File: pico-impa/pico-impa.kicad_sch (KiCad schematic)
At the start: 12 parts, among them J1 Barrel_Jack_MountingPin, U1 Pico, U2 Pico, U3 AMS1117-3.3

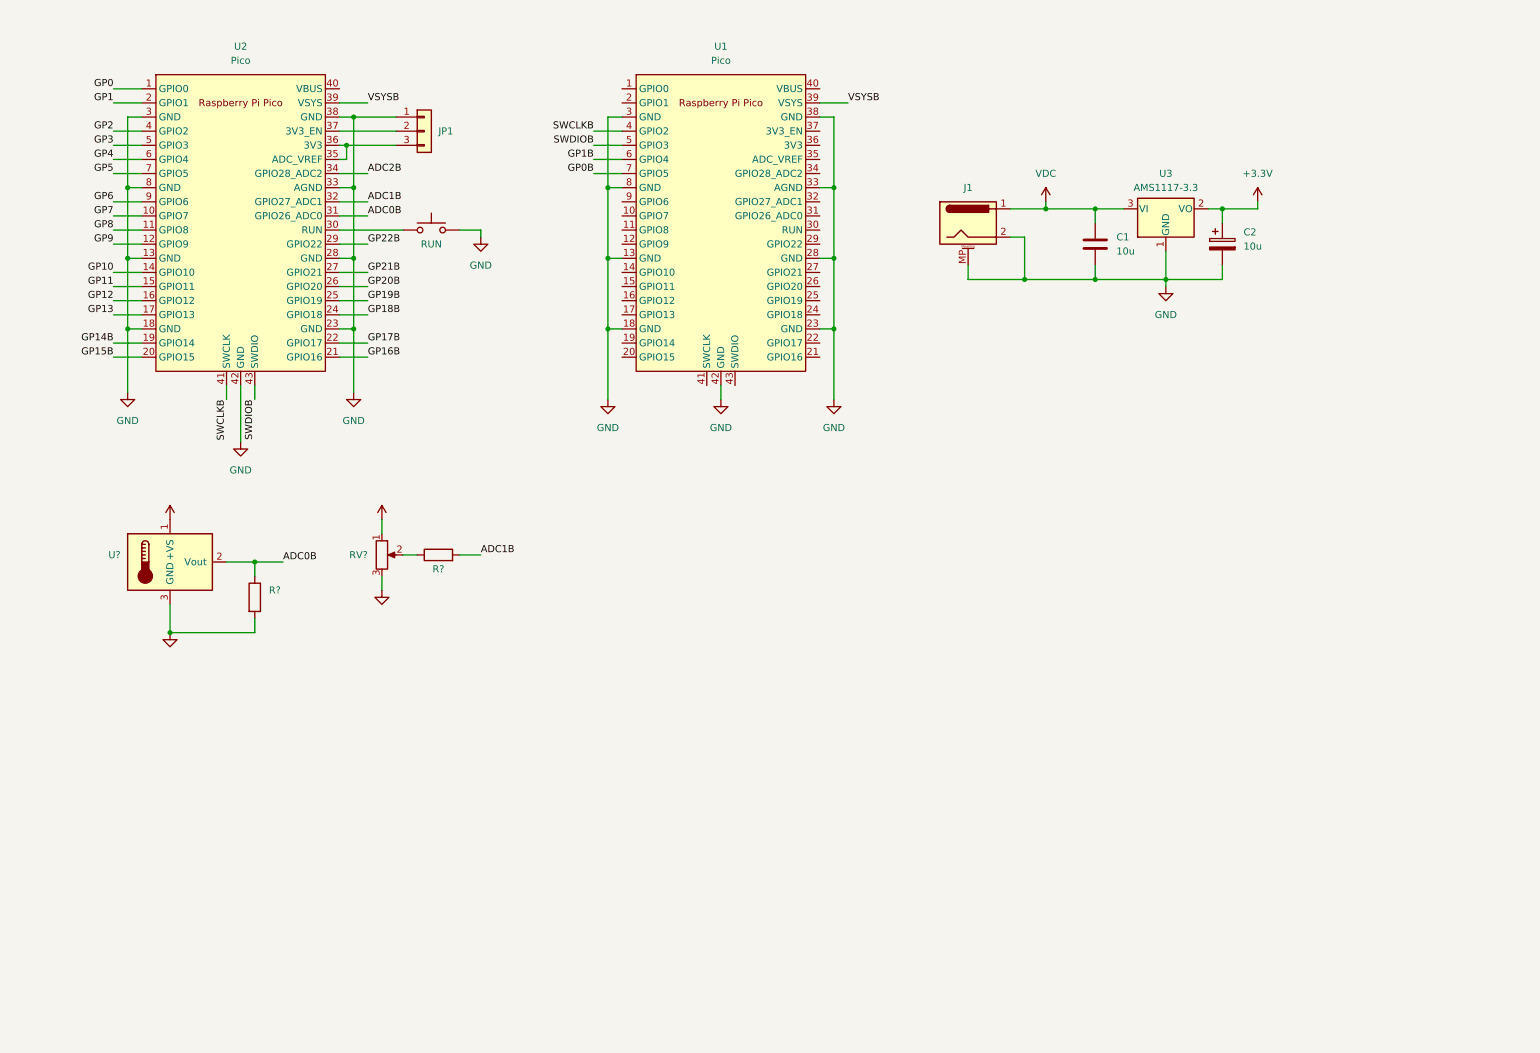
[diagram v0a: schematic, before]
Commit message: feat: first schematic version
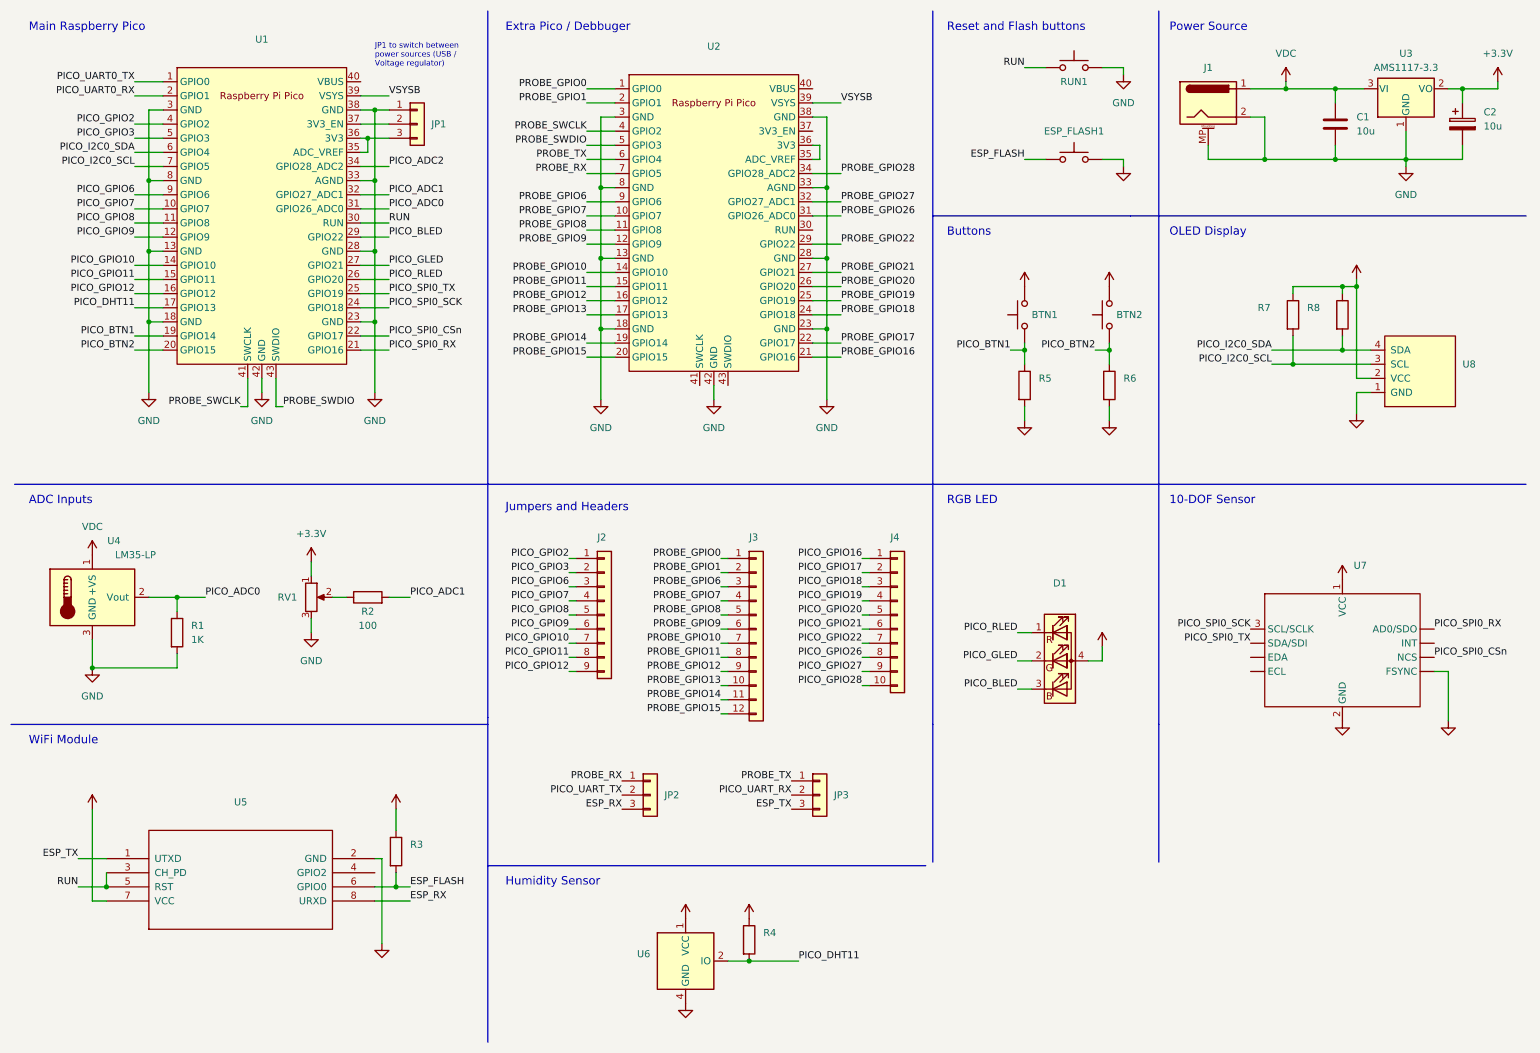
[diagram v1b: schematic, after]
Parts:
- added BTN1, BTN2, ESP_FLASH1: (no value), symbol Switch:SW_Push
- added D1: (no value), symbol Device:LED_RGBA
- added J2: (no value), symbol Connector_Generic:Conn_01x09
- added J3: (no value), symbol Connector_Generic:Conn_01x12
- added J4: (no value), symbol Connector_Generic:Conn_01x10
- added JP2, JP3: (no value), symbol Connector_Generic:Conn_01x03
- added R3, R4, R5, R6, R7, R8: (no value), symbol Device:R
- added U5: (no value), symbol ESP8266:ESP-01v090
- added U6: (no value), symbol Sensor:DHT11
- added U7: (no value), symbol Adafruit_Sensors:MPU9250
- added U8: (no value), symbol SSD1306-128x64_OLED:SSD1306
- R1: renamed from R?; value (none) -> 1K
- R2: renamed from R?; value (none) -> 100
- RV1: renamed from RV?; value (none) -> R_Potentiometer
- U1: renamed from U2; value Pico -> (none)
- U2: renamed from U1; value Pico -> (none)
- U4: renamed from U?; value (none) -> LM35-LP
- renumbered RUN to RUN1
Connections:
- net +3V3: now also BTN1.2, BTN2.2, D1.4 (A), R3.1, R4.1, R7.1, R8.1, U5.7 (VCC), U6.1 (VCC), U7.1 (VCC), U8.2 (VCC)
- net GND: now also ESP_FLASH1.2, R5.2, R6.2, U5.2 (GND), U6.4 (GND), U7. (SDA/SDI), U7.2 (GND), U8.1 (GND)
- net RUN: now reaches RUN1.1, U1.30 (RUN)
- net RUN: now also U5.3 (CH_PD), U5.5 (RST)
- net PROBE_GPIO0: now reaches U2.1 (GPIO0)
- net PROBE_GPIO0: now also J3.1 (Pin_1)
- net PROBE_GPIO7: now reaches U2.10 (GPIO7)
- net PROBE_GPIO7: now also J3.4 (Pin_4)
- net PROBE_GPIO8: now reaches U2.11 (GPIO8)
- net PROBE_GPIO8: now also J3.5 (Pin_5)
- net PROBE_GPIO9: now reaches U2.12 (GPIO9)
- net PROBE_GPIO9: now also J3.6 (Pin_6)
- net PROBE_GPIO10: now reaches U2.14 (GPIO10)
- net PROBE_GPIO10: now also J3.7 (Pin_7)
- net PROBE_GPIO11: now reaches U2.15 (GPIO11)
- net PROBE_GPIO11: now also J3.8 (Pin_8)
- net PROBE_GPIO12: now reaches U2.16 (GPIO12)
- net PROBE_GPIO12: now also J3.9 (Pin_9)
- net PROBE_GPIO13: now reaches U2.17 (GPIO13)
- net PROBE_GPIO13: now also J3.10 (Pin_10)
- net PROBE_GPIO14: now reaches U2.19 (GPIO14)
- net PROBE_GPIO14: now also J3.11 (Pin_11)
- net PROBE_GPIO1: now reaches U2.2 (GPIO1)
- net PROBE_GPIO1: now also J3.2 (Pin_2)
- net PROBE_GPIO15: now reaches U2.20 (GPIO15)
- net PROBE_GPIO15: now also J3.12 (Pin_12)
- net PROBE_GPIO16: now reaches U2.21 (GPIO16)
- net PROBE_GPIO17: now reaches U2.22 (GPIO17)
- net PROBE_GPIO18: now reaches U2.24 (GPIO18)
- net PROBE_GPIO19: now reaches U2.25 (GPIO19)
- net PROBE_GPIO20: now reaches U2.26 (GPIO20)
- net PROBE_GPIO21: now reaches U2.27 (GPIO21)
- net PROBE_GPIO22: now reaches U2.29 (GPIO22)
- net PROBE_GPIO26: now reaches U2.31 (GPIO26_ADC0)
- net PROBE_GPIO27: now reaches U2.32 (GPIO27_ADC1)
- net PROBE_GPIO28: now reaches U2.34 (GPIO28_ADC2)
- net at U2.35 (ADC_VREF): now also U2.36 (3V3)
- net PROBE_GPIO6: now reaches U2.9 (GPIO6)
- net PROBE_GPIO6: now also J3.3 (Pin_3)
- net ADC0B renamed PICO_ADC0
- net ADC1B renamed PICO_ADC1
- net ADC2B renamed PICO_ADC2
- net GP0 renamed PICO_UART0_TX
- net GP0B renamed PROBE_RX
- net PROBE_RX: now also JP2.1 (Pin_1)
- net GP1 renamed PICO_UART0_RX
- net GP10 renamed PICO_GPIO10
- net PICO_GPIO10: now also J2.7 (Pin_7)
- net GP11 renamed PICO_GPIO11
- net PICO_GPIO11: now also J2.8 (Pin_8)
- net GP12 renamed PICO_GPIO12
- net PICO_GPIO12: now also J2.9 (Pin_9)
- net GP13 renamed PICO_DHT11
- net PICO_DHT11: now also R4.2, U6.2 (IO)
- net GP14B renamed PICO_BTN1
- net PICO_BTN1: now also BTN1.1, R5.1
- net GP15B renamed PICO_BTN2
- net PICO_BTN2: now also BTN2.1, R6.1
- net GP16B renamed PICO_SPI0_RX
- net PICO_SPI0_RX: now also U7. (SDA/SDI)
- net GP17B renamed PICO_SPI0_CSn
- net PICO_SPI0_CSn: now also U7. (SDA/SDI)
- net GP18B renamed PICO_SPI0_SCK
- net PICO_SPI0_SCK: now also U7.3 (SCL/SCLK)
- net GP19B renamed PICO_SPI0_TX
- net PICO_SPI0_TX: now also U7. (SDA/SDI)
- net GP1B renamed PROBE_TX
- net PROBE_TX: now also JP3.1 (Pin_1)
- net GP2 renamed PICO_GPIO2
- net PICO_GPIO2: now also J2.1 (Pin_1)
- net GP20B renamed PICO_RLED
- net PICO_RLED: now also D1.1 (RK)
- net GP21B renamed PICO_GLED
- net PICO_GLED: now also D1.2 (GK)
- net GP22B renamed PICO_BLED
- net PICO_BLED: now also D1.3 (BK)
- net GP3 renamed PICO_GPIO3
- net PICO_GPIO3: now also J2.2 (Pin_2)
- net GP4 renamed PICO_I2C0_SDA
- net PICO_I2C0_SDA: now also R8.2, U8.4 (SDA)
- net GP5 renamed PICO_I2C0_SCL
- net PICO_I2C0_SCL: now also R7.2, U8.3 (SCL)
- net GP6 renamed PICO_GPIO6
- net PICO_GPIO6: now also J2.3 (Pin_3)
- net GP7 renamed PICO_GPIO7
- net PICO_GPIO7: now also J2.4 (Pin_4)
- net GP8 renamed PICO_GPIO8
- net PICO_GPIO8: now also J2.5 (Pin_5)
- net GP9 renamed PICO_GPIO9
- net PICO_GPIO9: now also J2.6 (Pin_6)
- net SWCLKB renamed PROBE_SWCLK
- net SWDIOB renamed PROBE_SWDIO
- new net ESP_FLASH: ESP_FLASH1.1, R3.2, U5.6 (GPIO0)
- new net ESP_RX: JP2.3 (Pin_3), U5.8 (URXD)
- new net ESP_TX: JP3.3 (Pin_3), U5.1 (UTXD)
- new net PICO_GPIO16: J4.1 (Pin_1)
- new net PICO_GPIO17: J4.2 (Pin_2)
- new net PICO_GPIO18: J4.3 (Pin_3)
- new net PICO_GPIO19: J4.4 (Pin_4)
- new net PICO_GPIO20: J4.5 (Pin_5)
- new net PICO_GPIO21: J4.6 (Pin_6)
- new net PICO_GPIO22: J4.7 (Pin_7)
- new net PICO_GPIO26: J4.8 (Pin_8)
- new net PICO_GPIO27: J4.9 (Pin_9)
- new net PICO_GPIO28: J4.10 (Pin_10)
- new net PICO_UART_RX: JP3.2 (Pin_2)
- new net PICO_UART_TX: JP2.2 (Pin_2)
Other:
- note added: "10-DOF Sensor"
- note added: "ADC Inputs"
- note added: "Buttons"
- note added: "Extra Pico / Debbuger"
- note added: "Humidity Sensor"
- note added: "JP1 to switch between power sources (USB / Voltage regulator)"
- note added: "Jumpers and Headers"
- note added: "Main Raspberry Pico"
- note added: "OLED Display"
- note added: "Power Source"
- note added: "RGB LED"
- note added: "Reset and Flash buttons"
- note added: "WiFi Module"
- moved on the sheet: C1, C2, J1, JP1, R1, R2, RUN1, RV1, U1, U2, U3, U4
